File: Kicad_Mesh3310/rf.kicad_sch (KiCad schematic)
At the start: 4 parts, among them U2 Ai-Thinker-Ra-01H

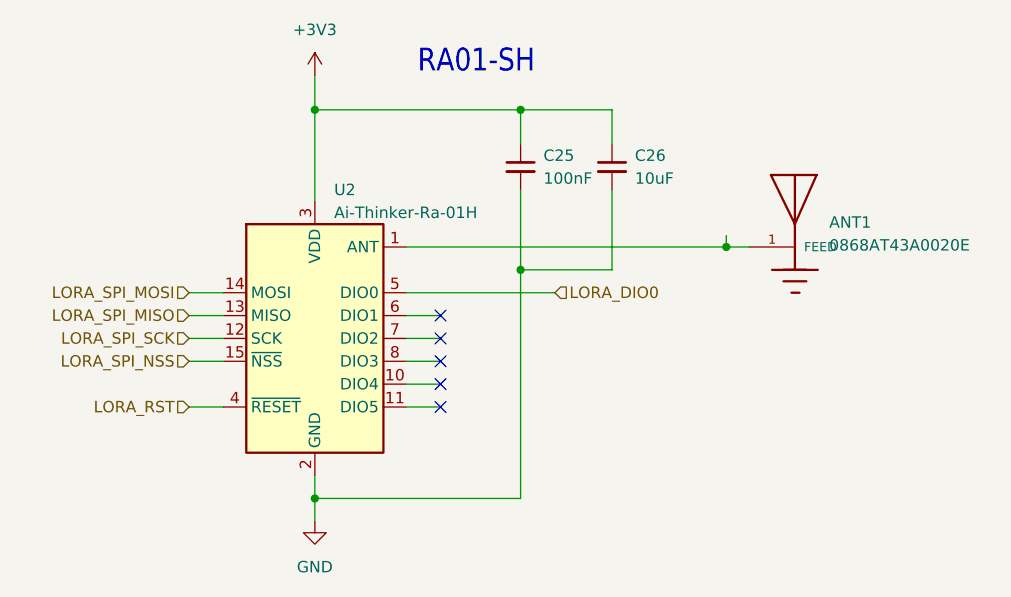
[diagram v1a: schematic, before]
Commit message: cleanup
schematic cleanup
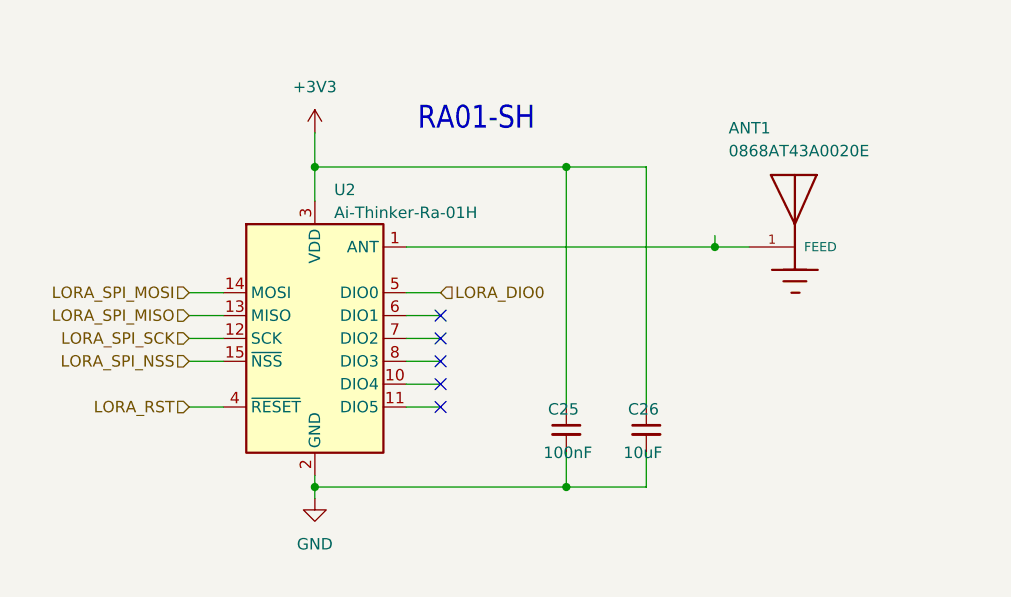
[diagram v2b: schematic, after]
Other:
- moved on the sheet: C25, C26
